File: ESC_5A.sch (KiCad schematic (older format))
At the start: 21 parts, among them IC1 ATSAMD21E17D-AUT, IC2 AP2112K-3.3TRG1, IC3 AP1501A-50K5G-13, J1 USB4105-GF-A, J2 Conn_01x03_Male, SW1 SW_Push

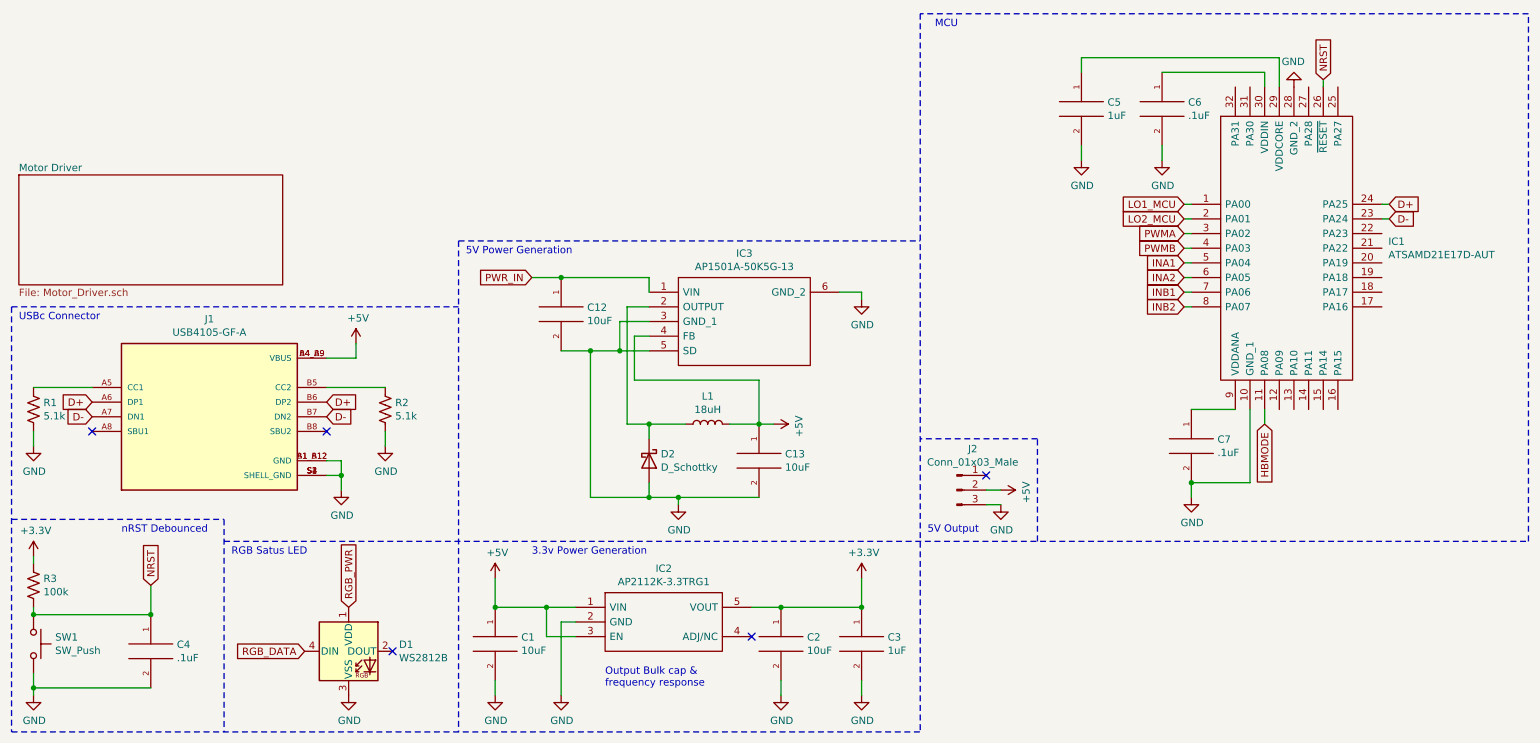
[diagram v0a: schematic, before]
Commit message: Schematic Rev_One Done pre review
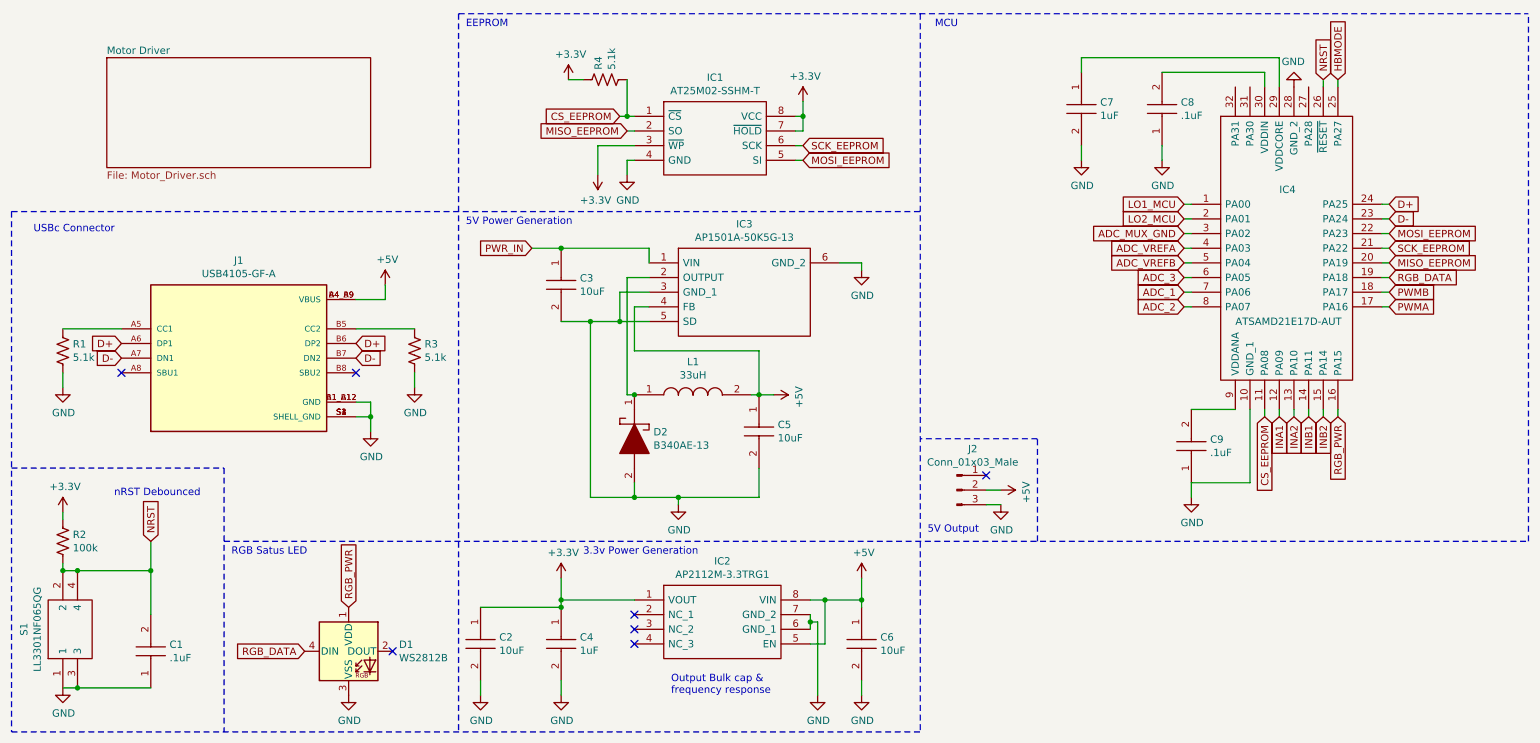
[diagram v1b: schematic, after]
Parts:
- removed C1, C12, C13, C2: 10uF, symbol pspice:CAP
- removed C3, C5: 1uF, symbol pspice:CAP
- removed C4, C6, C7: .1uF, symbol pspice:CAP
- removed D2: D_Schottky, symbol Device:D_Schottky
- removed IC2: AP2112K-3.3TRG1, SamacSys_Parts:SOT95P282X130-5N, symbol SamacSys_Parts:AP2112K-3.3TRG1
- removed L1: 18uH, symbol Device:L
- removed SW1: SW_Push, symbol Switch:SW_Push
- added C1, C8, C9: .1uF, SamacSys_Parts:CAPC0603X33N, symbol SamacSys_Parts:GRM033R61C104KE84D
- added C2, C5, C6: 10uF, SamacSys_Parts:C1608_Commercial, symbol SamacSys_Parts:C1608X5R1C106M080AB
- added C3: 10uF, SamacSys_Parts:CAPC3216X180N, symbol SamacSys_Parts:GRT31CR61H106KE01L
- added C4, C7: 1uF, SamacSys_Parts:CAPC1005X55N, symbol SamacSys_Parts:GRM155C81C105KE11J
- added D2: B340AE-13, SamacSys_Parts:DIOM5226X240N, symbol SamacSys_Parts:B340AE-13
- added IC1: AT25M02-SSHM-T, SamacSys_Parts:SOIC127P600X175-8N, symbol SamacSys_Parts:AT25M02-SSHM-T
- added IC2: AP2112M-3.3TRG1, SamacSys_Parts:SOIC127P600X170-8N, symbol SamacSys_Parts:AP2112M-3.3TRG1
- added L1: 33uH, SamacSys_Parts:SRR1260-150M, symbol SamacSys_Parts:SRR1260-330M
- added R4: 5.1k, Resistor_SMD:R_0402_1005Metric, symbol Device:R_US
- added S1: LL3301NF065QG, SamacSys_Parts:LL3301NF065QG, symbol SamacSys_Parts:LL3301NF065QG
- J2: footprint (none) -> Connector_PinHeader_2.54mm:PinHeader_1x03_P2.54mm_Vertical
- R1: footprint (none) -> Resistor_SMD:R_0402_1005Metric
- R2: renamed from R3; footprint (none) -> Resistor_SMD:R_0402_1005Metric
- R3: renamed from R2; footprint (none) -> Resistor_SMD:R_0402_1005Metric
- renumbered IC1 to IC4
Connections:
- net +3V3: now also C2.1, C4.1, IC1.3 (~WP), IC1.7 (~HOLD), IC1.8 (VCC), IC2.1 (VOUT), R4.1
- net +5V: now also C5.1, C6.1, IC2.5 (EN), IC2.8 (VIN), L1.2
- net GND: now also C1.1, C2.2, C3.2, C4.2, C5.2, C6.2, C7.2, C8.1, C9.1, D2.2, IC1.4 (GND), IC2.6 (GND_1), IC2.7 (GND_2), S1.1, S1.3
- net HBMODE: now also IC4.25 (PA27); no longer IC4.11 (PA08)
- net INA1: now also IC4.12 (PA09); no longer IC4.5 (PA04)
- net INA2: now also IC4.13 (PA10); no longer IC4.6 (PA05)
- net INB1: now also IC4.14 (PA11); no longer IC4.7 (PA06)
- net INB2: now also IC4.15 (PA14); no longer IC4.8 (PA07)
- net NRST: now also C1.2, S1.2, S1.4
- net PWMA: now also IC4.17 (PA16); no longer IC4.3 (PA02)
- net PWMB: now also IC4.18 (PA17); no longer IC4.4 (PA03)
- net PWR_IN: now also C3.1
- net RGB_DATA: now also IC4.19 (PA18)
- net RGB_PWR: now also IC4.16 (PA15)
- net MISO_EEPROM: now reaches IC4.20 (PA19)
- net MISO_EEPROM: now also IC1.2 (SO)
- net SCK_EEPROM: now reaches IC4.21 (PA22)
- net SCK_EEPROM: now also IC1.6 (SCK)
- net MOSI_EEPROM: now reaches IC4.22 (PA23)
- net MOSI_EEPROM: now also IC1.5 (SI)
- net at IC4.29 (VDDCORE): now also C7.1
- net at IC4.30 (VDDIN): now also C8.2
- net at IC4.9 (VDDANA): now also C9.2
- net at IC3.2 (OUTPUT): now also D2.1, L1.1
- new net ADC_1: IC4.7 (PA06)
- new net ADC_2: IC4.8 (PA07)
- new net ADC_3: IC4.6 (PA05)
- new net ADC_MUX_GND: IC4.3 (PA02)
- new net ADC_VREFA: IC4.4 (PA03)
- new net ADC_VREFB: IC4.5 (PA04)
- new net CS_EEPROM: IC1.1 (~CS), IC4.11 (PA08), R4.2
- no-connect marks 5 -> 7
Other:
- note added: "EEPROM"
- moved on the sheet: IC3, J1, R1, R2, R3
